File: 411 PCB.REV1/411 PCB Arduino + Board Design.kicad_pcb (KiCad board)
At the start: 2 copper layers, 42.1 x 62.6 mm, 28 parts, among them J1 ICSP CONN, J2 Conn_01x06_MountingPin, J4 Conn_01x04, Q1 Q_NMOS_GDS, SW1 SW_SPST, SW3 SW_MEC_5E, U1 ATmega328P-P, Y1 8 MHz

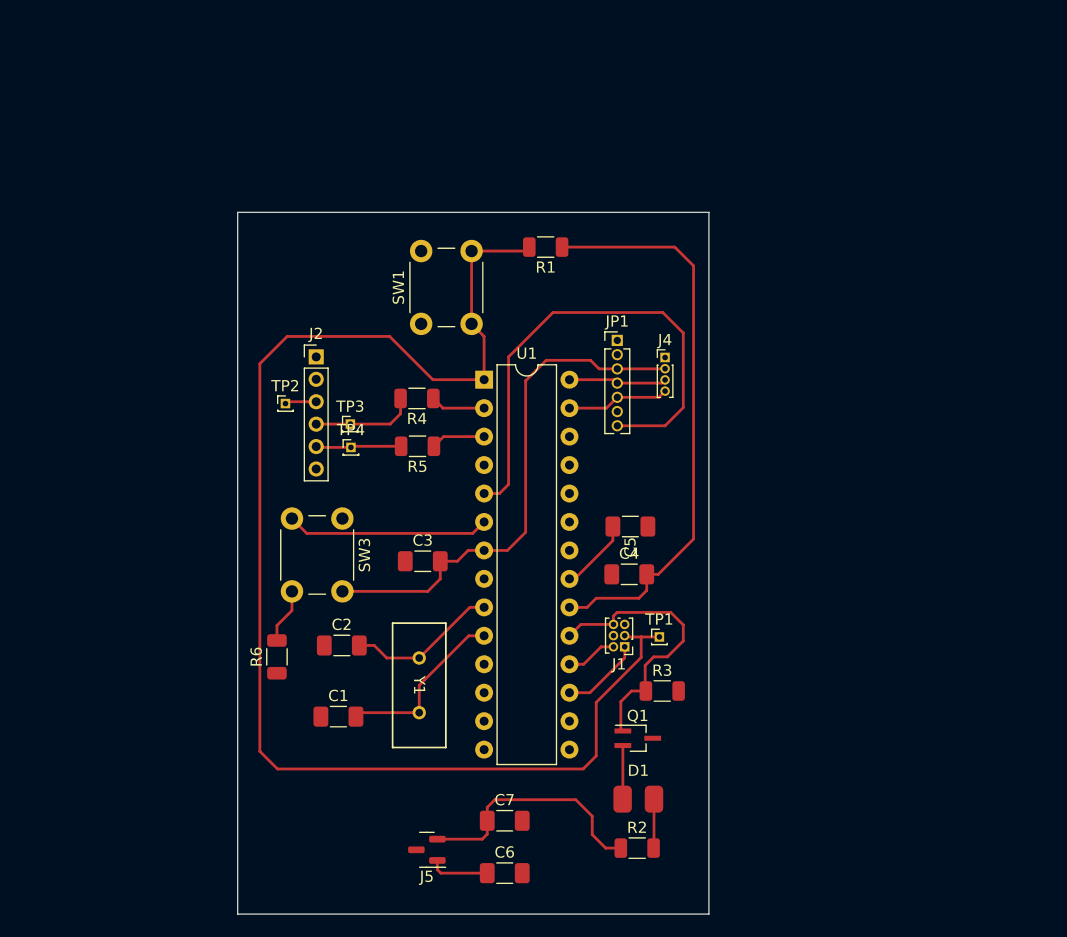
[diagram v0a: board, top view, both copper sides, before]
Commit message: update
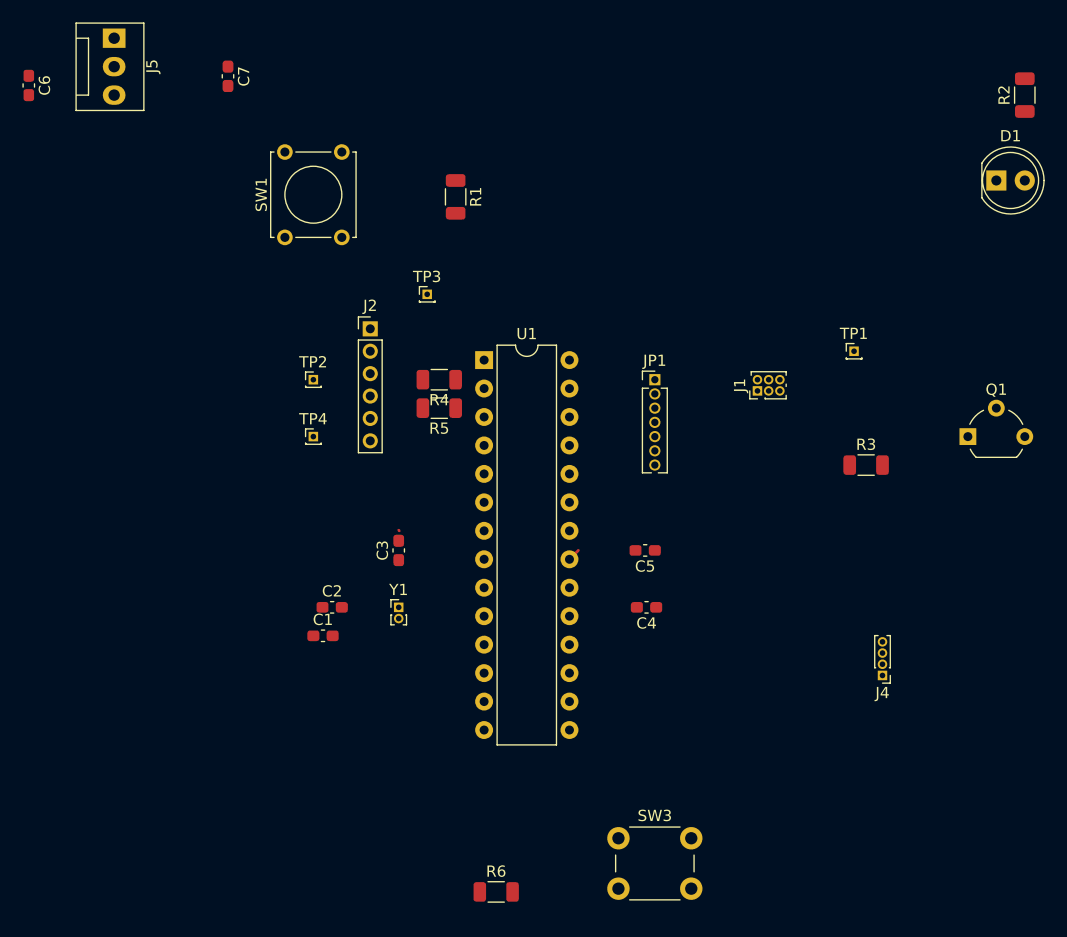
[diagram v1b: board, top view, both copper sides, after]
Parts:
- C1, C2, C3, C4, C5, C6, C7: footprint Capacitor_SMD:C_1206_3216Metric_Pad1.33x1.80mm_HandSolder -> Capacitor_SMD:C_0603_1608Metric_Pad1.08x0.95mm_HandSolder
- D1: footprint LED_SMD:LED_0805_2012Metric_Pad1.15x1.40mm_HandSolder -> LED_THT:LED_D5.0mm_Clear
- J5: footprint Package_TO_SOT_SMD:SOT-23 -> Connector:FanPinHeader_1x03_P2.54mm_Vertical
- Q1: footprint Package_TO_SOT_SMD:SOT-323_SC-70_Handsoldering -> Package_TO_SOT_THT:TO-92_Wide
- SW1: footprint Button_Switch_THT:SW_PUSH_6mm -> Button_Switch_THT:SW_Tactile_Straight_KSA0Axx1LFTR
- SW3: footprint Button_Switch_THT:SW_PUSH_6mm -> Button_Switch_THT:SW_PUSH_6mm_H4.3mm
- Y1: footprint footprints:ATS08A-E_CTS -> Connector_PinHeader_1.00mm:PinHeader_1x02_P1.00mm_Vertical
- moved C6 82.1 mm to (119.4, 42.3), turned to -90 degrees
- moved J5 77.6 mm to (127.0, 38.1), turned to -90 degrees
- moved R2 75.6 mm to (208.3, 43.2), turned to 90 degrees
- moved C7 70.9 mm to (137.2, 41.5), turned to -90 degrees
- moved D1 63.8 mm to (205.7, 50.8)
- moved Q1 39.9 mm to (203.2, 73.7)
- moved SW3 37.7 mm to (172.0, 109.5), turned to 0 degrees
- moved J4 34.4 mm to (195.6, 95.0), turned to 180 degrees
- moved TP1 30.9 mm to (193.0, 66.0)
- moved R6 28.7 mm to (161.1, 114.3), turned to 0 degrees
- moved R3 27.2 mm to (194.1, 76.2)
- moved J1 25.7 mm to (184.4, 69.6), turned to 90 degrees
- moved SW1 14.4 mm to (142.2, 55.9)
- moved TP3 13.5 mm to (154.9, 61.0)
- moved R1 9.20 mm to (157.5, 52.3), turned to -90 degrees
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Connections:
- SW3 pad 2: Net-(R6-Pad2) -> +3.3V
- SW3 pad 3: unconnected-(SW3-K-Pad3) -> Net-(R6-Pad2)
- SW3 pad 4: Net-(SW3-A) -> Net-(R6-Pad2)
- U1 pad 12: unconnected-(U1-(AIN0)PD6-Pad12) -> /LED_EN
- U1 pad 13: unconnected-(U1-(AIN1)PD7-Pad13) -> Net-(SW3-A)
- U1 pad 5: /LED_EN -> unconnected-(U1-(INT1)PD3-Pad5)
- U1 pad 6: Net-(SW3-A) -> unconnected-(U1-(T0)PD4-Pad6)
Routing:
- net Net-(J1-~{RST}): track 121.0 -> 0.00 mm
- net +3.3V: track 119.7 -> 0.07 mm
- net /LED_EN: track 45.1 -> 0.00 mm
- net Net-(J1-SCK): track 25.3 -> 0.00 mm
- net Net-(SW3-A): track 18.1 -> 0.00 mm
- net Net-(U1-XTAL2/PB7): track 15.9 -> 0.00 mm
- net Net-(U1-XTAL1/PB6): track 13.5 -> 0.00 mm
- net Net-(J2-Pin_4): track 9.28 -> 0.00 mm
- net /SDA_3.3V: track 9.16 -> 0.00 mm
- net /SCL_3.3V: track 8.78 -> 0.00 mm
- net Net-(J2-Pin_5): track 7.65 -> 0.00 mm
- net Net-(J1-MOSI): track 7.21 -> 0.00 mm
- net Net-(U1-AREF): track 6.55 -> 1.12 mm
- net +VDC: track 5.40 -> 0.00 mm
- net Net-(R6-Pad2): track 4.94 -> 0.00 mm
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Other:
- board outline removed
